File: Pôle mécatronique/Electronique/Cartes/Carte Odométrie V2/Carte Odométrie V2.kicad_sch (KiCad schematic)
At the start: 30 parts, among them J1 X2, J2 X1, J3 X3, U1 MCP2551-I-P

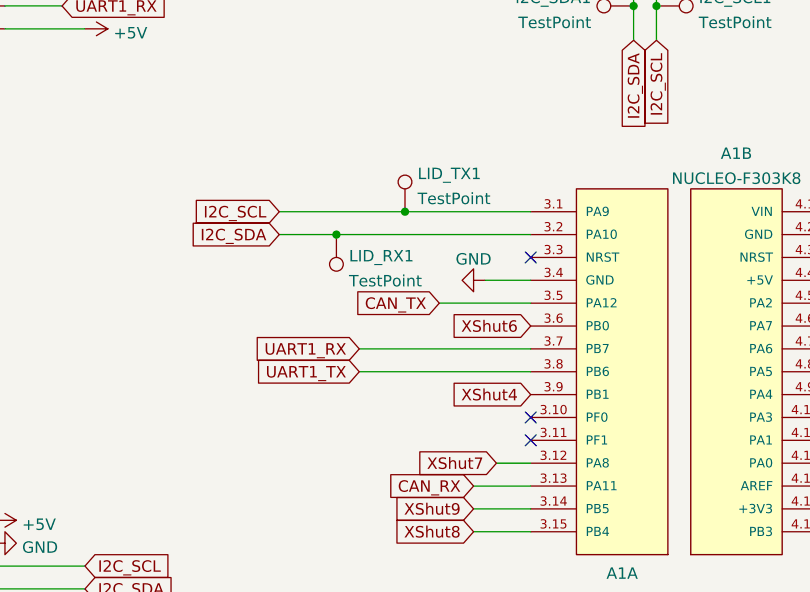
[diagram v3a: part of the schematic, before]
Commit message: OUHO
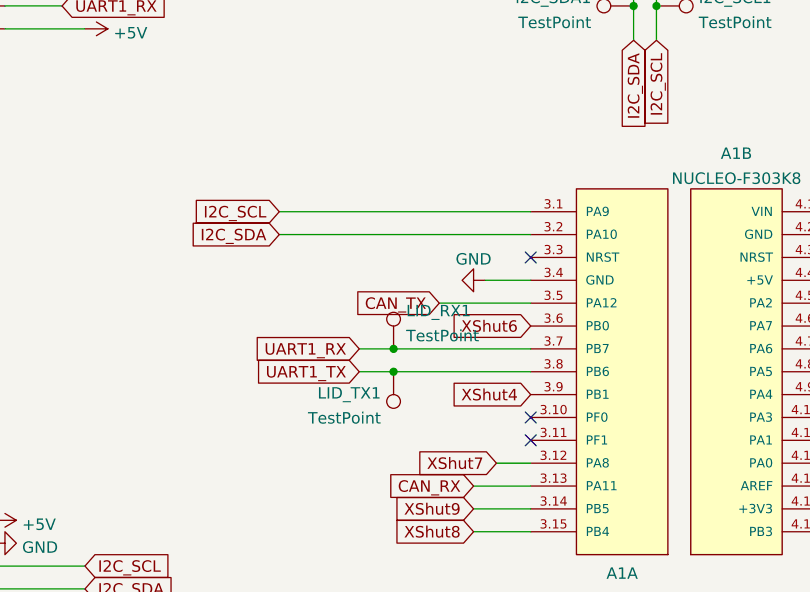
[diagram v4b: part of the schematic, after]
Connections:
- net I2C_SCL: no longer LID_TX1.1
- net I2C_SDA: no longer LID_RX1.1
- net UART1_RX: now also LID_RX1.1
- net UART1_TX: now also LID_TX1.1
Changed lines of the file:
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@@
   (junction (at 135.89 38.1) (diameter 0) (color 0 0 0 0)
   )
-  (junction (at 102.87 63.5) (diameter 0) (color 0 0 0 0)
-  )
   (junction (at 167.64 62.23) (diameter 0) (color 0 0 0 0)
   )
   (junction (at 165.1 135.89) (diameter 0) (color 0 0 0 0)
   )
-  (junction (at 110.49 60.96) (diameter 0) (color 0 0 0 0)
-  )
   (junction (at 127 134.62) (diameter 0) (color 0 0 0 0)
   )
@@
   (junction (at 199.39 93.98) (diameter 0) (color 0 0 0 0)
   )
+  (junction (at 109.22 76.2) (diameter 0) (color 0 0 0 0)
+  )
   (junction (at 167.64 69.85) (diameter 0) (color 0 0 0 0)
   )
@@
   )
   (junction (at 173.99 62.23) (diameter 0) (color 0 0 0 0)
+  )
+  (junction (at 109.22 78.74) (diameter 0) (color 0 0 0 0)
   )
   (no_connect (at 125.73 142.24))
@@
     (stroke (width 0) (type default) (color 0 0 0 0))
   )
-  (wire (pts (xy 105.41 78.74) (xy 124.46 78.74))
+  (wire (pts (xy 105.41 78.74) (xy 109.22 78.74))
     (stroke (width 0) (type default) (color 0 0 0 0))
   )
@@
     (stroke (width 0) (type default) (color 0 0 0 0))
   )
+  (wire (pts (xy 109.22 78.74) (xy 124.46 78.74))
+    (stroke (width 0) (type default) (color 0 0 0 0))
+  )
   (wire (pts (xy 66.04 35.56) (xy 72.39 35.56))
     (stroke (width 0) (type default) (color 0 0 0 0))
@@
     (stroke (width 0) (type default) (color 0 0 0 0))
   )
-  (wire (pts (xy 102.87 63.5) (xy 124.46 63.5))
+  (wire (pts (xy 109.22 76.2) (xy 105.41 76.2))
     (stroke (width 0) (type default) (color 0 0 0 0))
   )
@@
     (stroke (width 0) (type default) (color 0 0 0 0))
   )
-  (wire (pts (xy 124.46 76.2) (xy 105.41 76.2))
+  (wire (pts (xy 124.46 76.2) (xy 109.22 76.2))
     (stroke (width 0) (type default) (color 0 0 0 0))
   )
@@
     (stroke (width 0) (type default) (color 0 0 0 0))
   )
-  (wire (pts (xy 110.49 60.96) (xy 124.46 60.96))
-    (stroke (width 0) (type default) (color 0 0 0 0))
-  )
   (wire (pts (xy 157.48 137.16) (xy 157.48 135.89))
     (stroke (width 0) (type default) (color 0 0 0 0))
@@
     (stroke (width 0) (type default) (color 0 0 0 0))
   )
-  (wire (pts (xy 96.52 63.5) (xy 102.87 63.5))
+  (wire (pts (xy 96.52 63.5) (xy 124.46 63.5))
     (stroke (width 0) (type default) (color 0 0 0 0))
   )
@@
     (stroke (width 0) (type default) (color 0 0 0 0))
   )
-  (wire (pts (xy 96.52 60.96) (xy 110.49 60.96))
+  (wire (pts (xy 96.52 60.96) (xy 124.46 60.96))
     (stroke (width 0) (type default) (color 0 0 0 0))
   )
@@
       (effects (font (size 1.27 1.27)) (justify left) hide)
     )
-  )
-  (symbol (lib_id "Connector:TestPoint") (at 110.49 60.96 0) (unit 1)
-    (in_bom yes) (on_board yes) (fields_autoplaced)
-    (property "Reference" "LID_TX1" (id 0) (at 111.887 56.7495 0)
-      (effects (font (size 1.27 1.27)) (justify left))
-    )
-    (property "Value" "TestPoint" (id 1) (at 111.887 59.5246 0)
-      (effects (font (size 1.27 1.27)) (justify left))
-    )
-    (property "Footprint" "TestPoint:TestPoint_Pad_D2.0mm" (id 2) (at 115.57 60.96 0)
-      (effects (font (size 1.27 1.27)) hide)
-    )
-    (property "Datasheet" "~" (id 3) (at 115.57 60.96 0)
-      (effects (font (size 1.27 1.27)) hide)
-    )
-    (pin "1")
   )
   (symbol (lib_id "Connector_Generic:Conn_01x05") (at 60.96 35.56 0) (mirror y) (unit 1)
@@
     (pin "1")
   )
+  (symbol (lib_id "Connector:TestPoint") (at 109.22 78.74 0) (mirror x) (unit 1)
+    (in_bom yes) (on_board yes) (fields_autoplaced)
+    (property "Reference" "LID_TX1" (id 0) (at 107.823 81.1335 0)
+      (effects (font (size 1.27 1.27)) (justify right))
+    )
+    (property "Value" "TestPoint" (id 1) (at 107.823 83.9086 0)
+      (effects (font (size 1.27 1.27)) (justify right))
+    )
+    (property "Footprint" "TestPoint:TestPoint_Pad_D2.0mm" (id 2) (at 114.3 78.74 0)
+      (effects (font (size 1.27 1.27)) hide)
+    )
+    (property "Datasheet" "~" (id 3) (at 114.3 78.74 0)
+      (effects (font (size 1.27 1.27)) hide)
+    )
+    (pin "1")
+  )
+  (symbol (lib_id "Connector:TestPoint") (at 109.22 76.2 0) (mirror y) (unit 1)
+    (in_bom yes) (on_board yes) (fields_autoplaced)
+    (property "Reference" "LID_RX1" (id 0) (at 110.617 71.9895 0)
+      (effects (font (size 1.27 1.27)) (justify right))
+    )
+    (property "Value" "TestPoint" (id 1) (at 110.617 74.7646 0)
+      (effects (font (size 1.27 1.27)) (justify right))
+    )
+    (property "Footprint" "TestPoint:TestPoint_Pad_D2.0mm" (id 2) (at 104.14 76.2 0)
+      (effects (font (size 1.27 1.27)) hide)
+    )
+    (property "Datasheet" "~" (id 3) (at 104.14 76.2 0)
+      (effects (font (size 1.27 1.27)) hide)
+    )
+    (pin "1")
+  )
   (symbol (lib_id "power:+5V") (at 227.33 86.36 90) (mirror x) (unit 1)
     (in_bom yes) (on_board yes) (fields_autoplaced)
@@
     (pin "1")
   )
-  (symbol (lib_id "Connector:TestPoint") (at 102.87 63.5 180) (unit 1)
-    (in_bom yes) (on_board yes) (fields_autoplaced)
-    (property "Reference" "LID_RX1" (id 0) (at 104.267 65.8935 0)
-      (effects (font (size 1.27 1.27)) (justify right))
-    )
-    (property "Value" "TestPoint" (id 1) (at 104.267 68.6686 0)
-      (effects (font (size 1.27 1.27)) (justify right))
-    )
-    (property "Footprint" "TestPoint:TestPoint_Pad_D2.0mm" (id 2) (at 97.79 63.5 0)
-      (effects (font (size 1.27 1.27)) hide)
-    )
-    (property "Datasheet" "~" (id 3) (at 97.79 63.5 0)
-      (effects (font (size 1.27 1.27)) hide)
-    )
-    (pin "1")
-  )
   (symbol (lib_id "Connector_Generic:Conn_01x04") (at 237.49 36.83 0) (unit 1)
     (in_bom yes) (on_board yes) (fields_autoplaced)
@@
       (reference "LIDAR1") (unit 1) (value "Conn_01x05") (footprint "Connector_JST:JST_PH_B5B-PH-K_1x05_P2.00mm_Vertical")
     )
-    (path "/ebce3722-e17c-409e-9360-70d62b4f134f"
+    (path "/ae9affef-b25d-4f38-ae2b-90f62540bf33"
       (reference "LID_RX1") (unit 1) (value "TestPoint") (footprint "TestPoint:TestPoint_Pad_D2.0mm")
     )
-    (path "/009b18b2-25ab-4394-b7f1-0e9c8ad25691"
+    (path "/ae4aa54e-a780-4e26-8a76-8295f04ee892"
       (reference "LID_TX1") (unit 1) (value "TestPoint") (footprint "TestPoint:TestPoint_Pad_D2.0mm")
     )

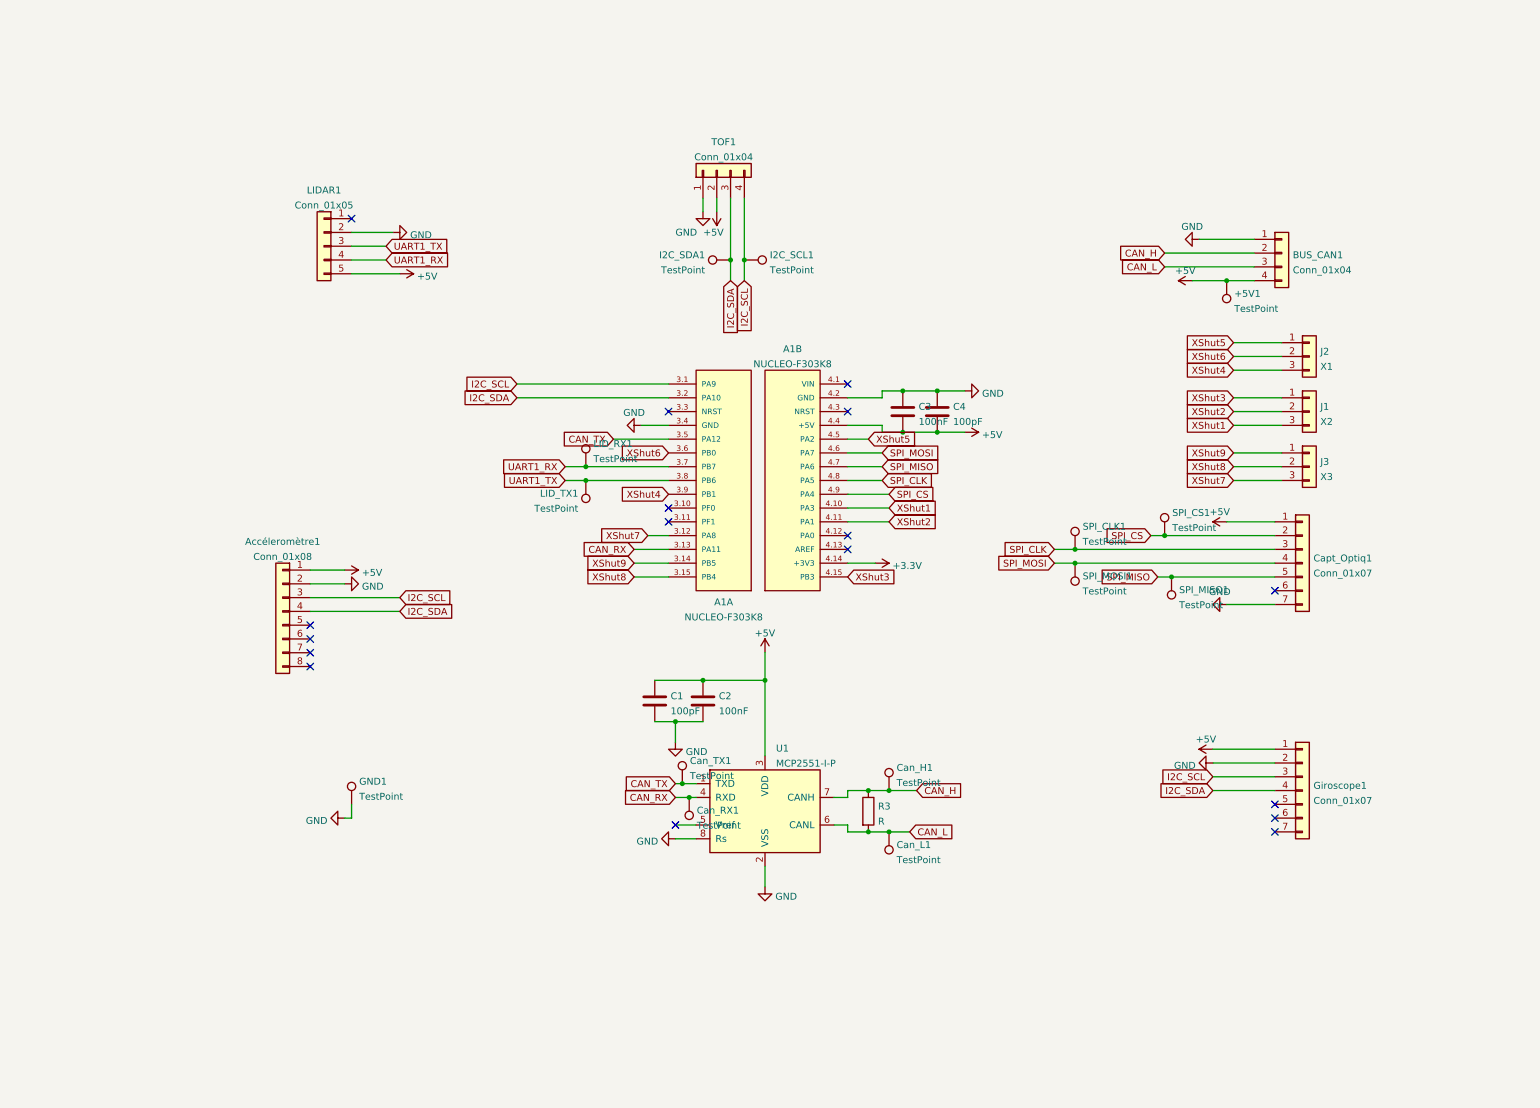
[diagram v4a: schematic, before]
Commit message: pin out
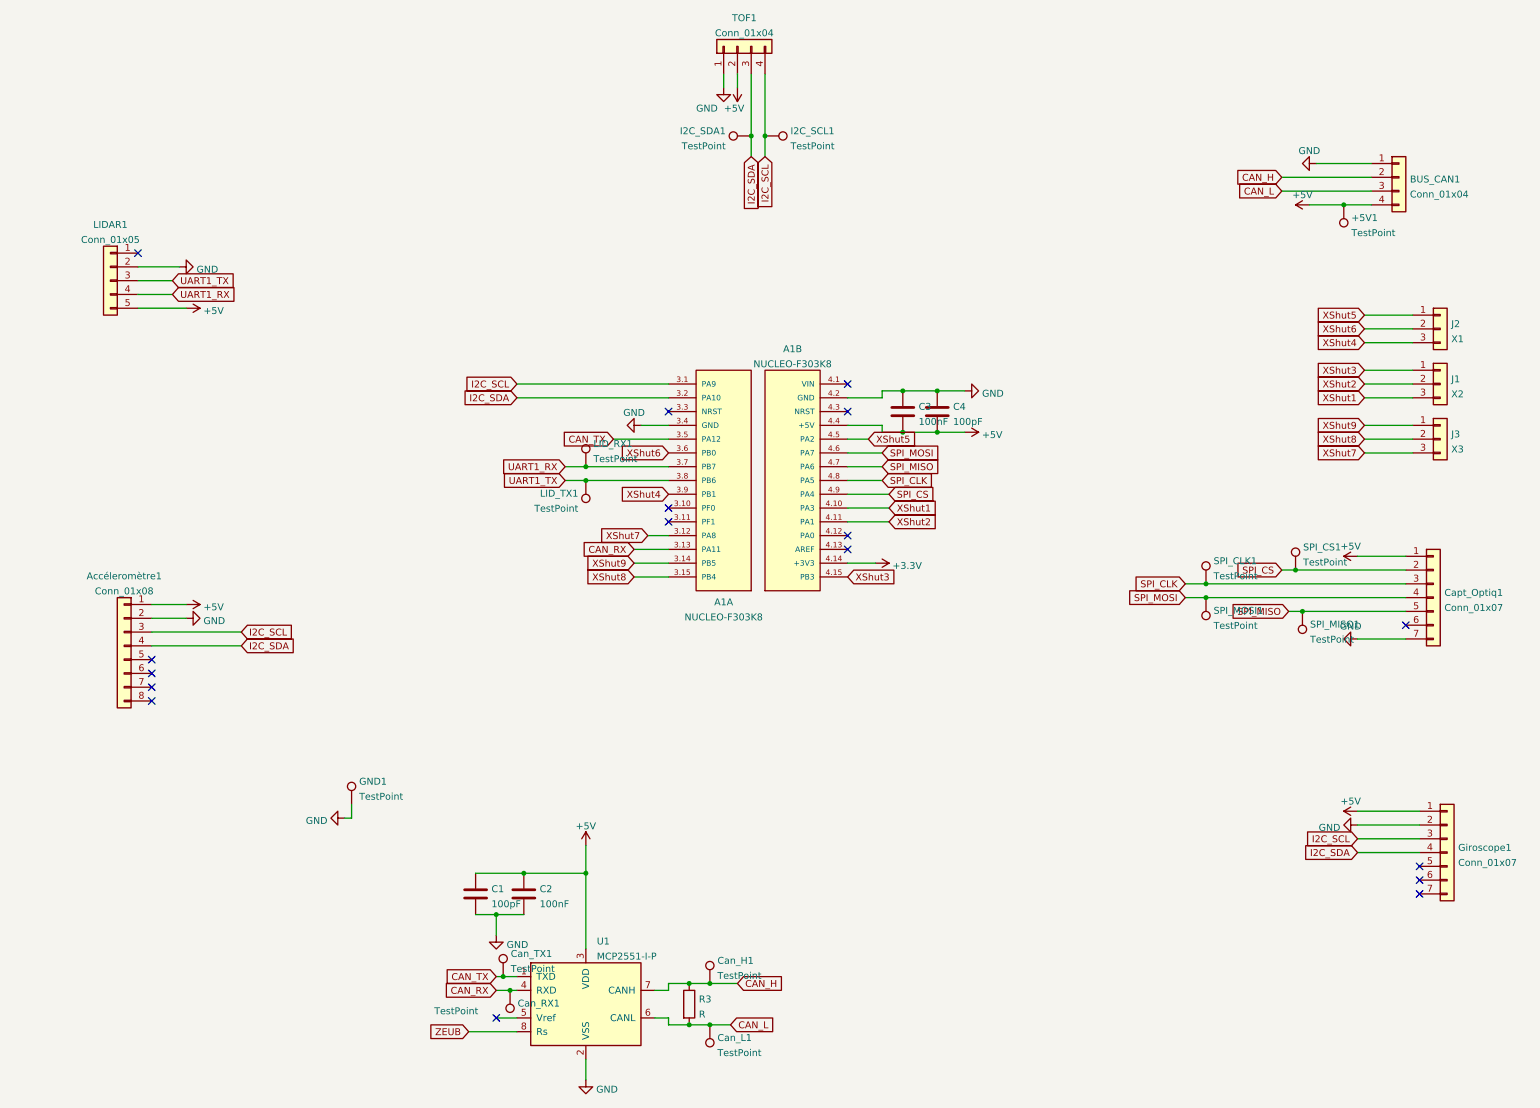
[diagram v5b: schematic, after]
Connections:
- net GND: no longer U1.8 (Rs)
- new net ZEUB: U1.8 (Rs)
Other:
- moved on the sheet: +5V1, Accéleromètre1, BUS_CAN1, C1, C2, Can_H1, Can_L1, Can_RX1, Can_TX1, Capt_Optiq1, Giroscope1, I2C_SCL1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

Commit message: Updateu
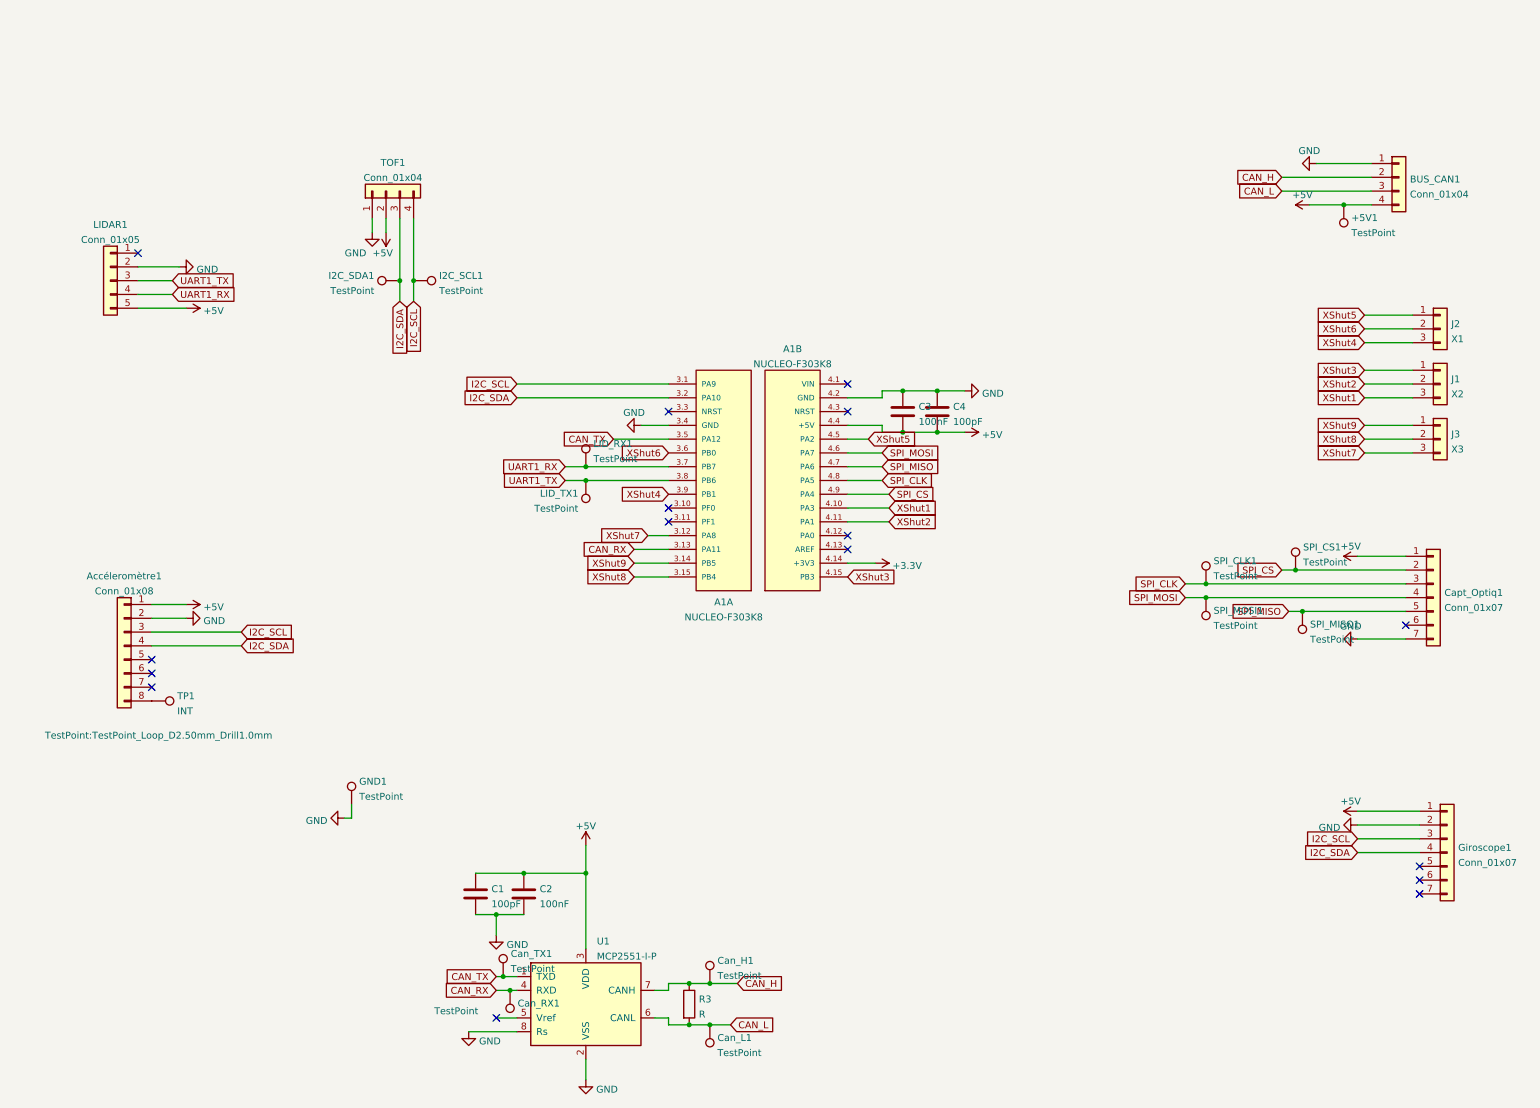
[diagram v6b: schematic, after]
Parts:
- added TP1: INT, TestPoint:TestPoint_Loop_D2.50mm_Drill1.0mm, symbol Connector:TestPoint
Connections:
- net ZEUB is gone; now on net GND: U1.8 (Rs)
- net at Accéleromètre1.8 (Pin_8): now also TP1.1
- no-connect marks 17 -> 16
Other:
- moved on the sheet: I2C_SCL1, I2C_SDA1, TOF1
